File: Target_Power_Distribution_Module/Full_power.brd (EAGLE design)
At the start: 64.4 x 39.4 mm, 28 parts, among them IC1 MCP1702, Q1 NFET, Q2 PFET, Q3 NFET, Q4 PFET

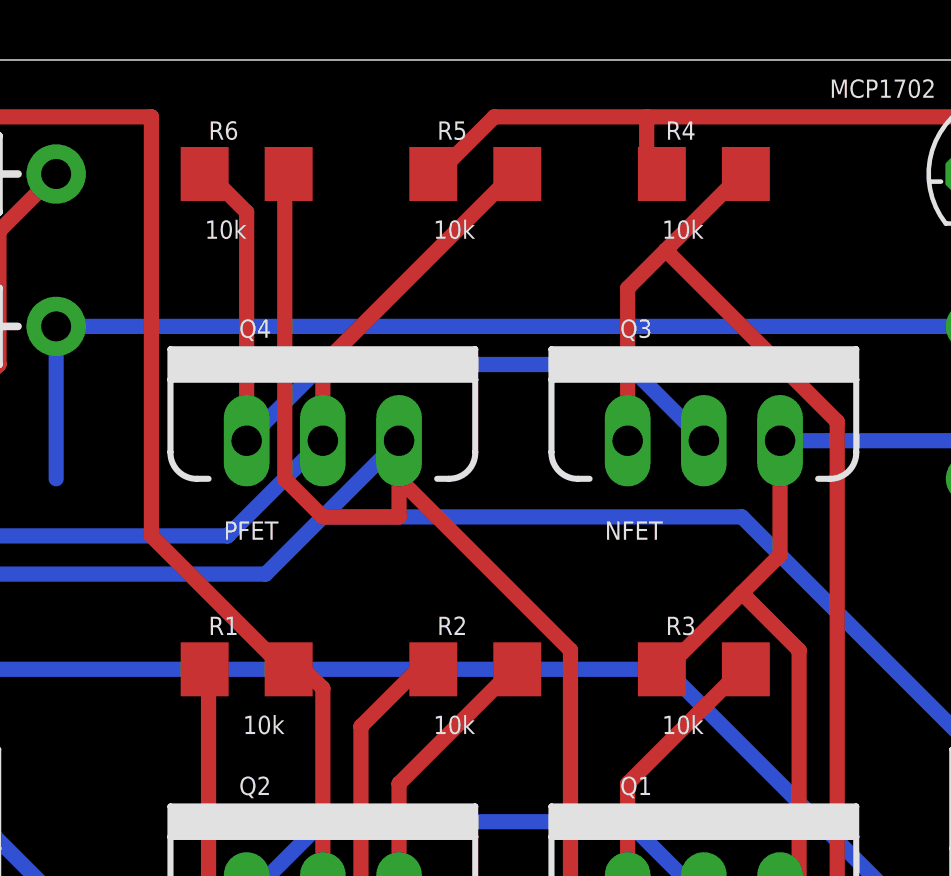
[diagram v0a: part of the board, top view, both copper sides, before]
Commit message: Cleaned sensor on full schem
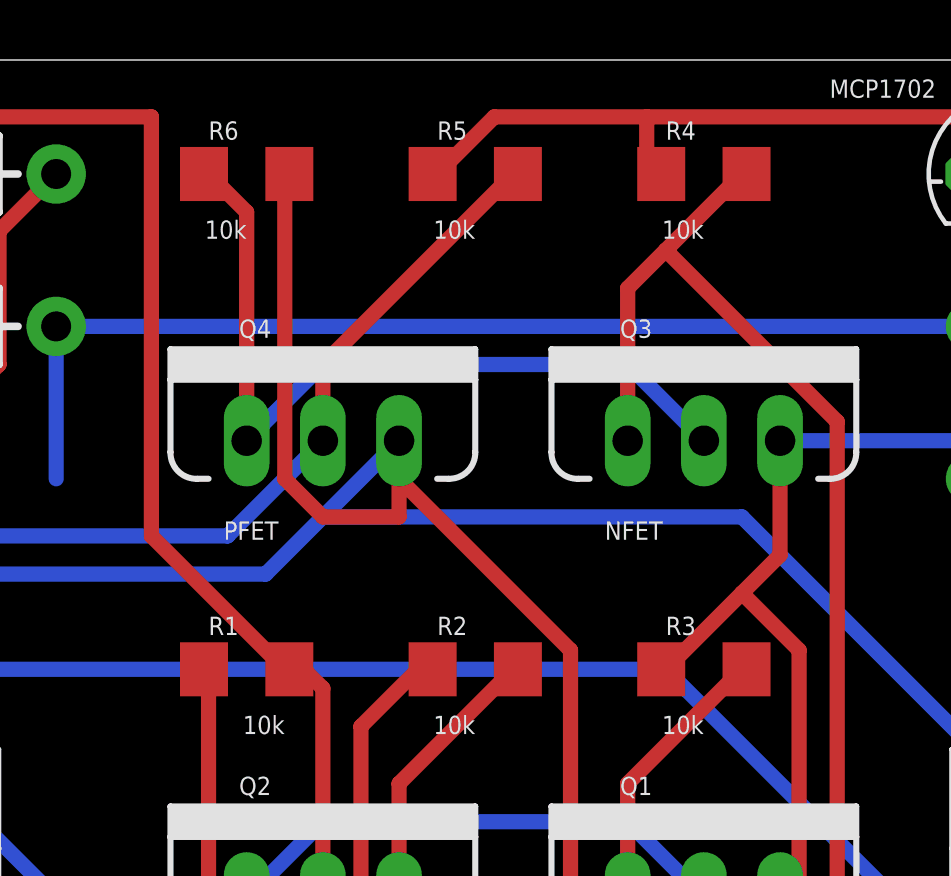
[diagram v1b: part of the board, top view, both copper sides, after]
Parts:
- R1, R2, R3, R4, R5, R6: device SparkFun-Resistors:1206 -> adafruit:R1206
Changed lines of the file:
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@@
 <attribute name="VALUE" x="33.528" y="64.008" size="0.6096" layer="25" ratio="10"/>
 </element>
-<element name="R1" library="SparkFun-Resistors" package="1206" value="10k" x="34.29" y="59.69" smashed="yes">
+<element name="R1" library="adafruit" package="R1206" value="10k" x="34.29" y="59.69" smashed="yes">
 <attribute name="NAME" x="33.02" y="60.833" size="0.6096" layer="25"/>
 <attribute name="VALUE" x="34.163" y="57.531" size="0.6096" layer="25"/>
 </element>
-<element name="R2" library="SparkFun-Resistors" package="1206" value="10k" x="41.91" y="59.69" smashed="yes">
+<element name="R2" library="adafruit" package="R1206" value="10k" x="41.91" y="59.69" smashed="yes">
 <attribute name="NAME" x="40.64" y="60.833" size="0.6096" layer="25"/>
 <attribute name="VALUE" x="40.513" y="57.531" size="0.6096" layer="25"/>
 </element>
-<element name="R3" library="SparkFun-Resistors" package="1206" value="10k" x="49.53" y="59.69" smashed="yes">
+<element name="R3" library="adafruit" package="R1206" value="10k" x="49.53" y="59.69" smashed="yes">
 <attribute name="NAME" x="48.26" y="60.833" size="0.6096" layer="25"/>
 <attribute name="VALUE" x="48.133" y="57.531" size="0.6096" layer="25"/>
 </element>
-<element name="R4" library="SparkFun-Resistors" package="1206" value="10k" x="49.53" y="76.2" smashed="yes">
+<element name="R4" library="adafruit" package="R1206" value="10k" x="49.53" y="76.2" smashed="yes">
 <attribute name="NAME" x="48.26" y="77.343" size="0.6096" layer="25"/>
 <attribute name="VALUE" x="48.133" y="74.041" size="0.6096" layer="25"/>
 </element>
-<element name="R5" library="SparkFun-Resistors" package="1206" value="10k" x="41.91" y="76.2" smashed="yes">
+<element name="R5" library="adafruit" package="R1206" value="10k" x="41.91" y="76.2" smashed="yes">
 <attribute name="NAME" x="40.64" y="77.343" size="0.6096" layer="25"/>
 <attribute name="VALUE" x="40.513" y="74.041" size="0.6096" layer="25"/>
 </element>
-<element name="R6" library="SparkFun-Resistors" package="1206" value="10k" x="34.29" y="76.2" smashed="yes">
+<element name="R6" library="adafruit" package="R1206" value="10k" x="34.29" y="76.2" smashed="yes">
 <attribute name="NAME" x="33.02" y="77.343" size="0.6096" layer="25"/>
 <attribute name="VALUE" x="32.893" y="74.041" size="0.6096" layer="25"/>
@@
 <wire x1="33.02" y1="48.26" x2="33.02" y2="59.69" width="0.508" layer="1"/>
 <wire x1="38.1" y1="43.18" x2="33.02" y2="48.26" width="0.508" layer="1"/>
-<wire x1="33.02" y1="59.69" x2="32.89" y2="59.69" width="0.508" layer="1"/>
+<wire x1="33.02" y1="59.69" x2="32.868" y2="59.69" width="0.508" layer="1"/>
 <wire x1="33.02" y1="46.355" x2="22.86" y2="46.355" width="0.508" layer="1"/>
 <wire x1="33.02" y1="48.26" x2="33.02" y2="46.355" width="0.508" layer="1"/>
@@
 <wire x1="50.8" y1="62.23" x2="48.26" y2="59.69" width="0.508" layer="1"/>
 <wire x1="52.07" y1="67.31" x2="52.07" y2="63.5" width="0.508" layer="1"/>
-<wire x1="48.26" y1="59.69" x2="48.13" y2="59.69" width="0.508" layer="1"/>
+<wire x1="48.26" y1="59.69" x2="48.108" y2="59.69" width="0.508" layer="1"/>
 <wire x1="52.705" y1="43.815" x2="52.705" y2="51.435" width="0.508" layer="1"/>
 <wire x1="53.34" y1="43.18" x2="52.705" y2="43.815" width="0.508" layer="1"/>
@@
 <wire x1="47.625" y1="78.105" x2="42.545" y2="78.105" width="0.508" layer="1"/>
 <wire x1="47.625" y1="76.2" x2="47.625" y2="78.105" width="0.508" layer="1"/>
-<wire x1="40.64" y1="76.2" x2="40.51" y2="76.2" width="0.508" layer="1"/>
-<wire x1="47.625" y1="76.2" x2="48.13" y2="76.2" width="0.508" layer="1"/>
+<wire x1="40.64" y1="76.2" x2="40.488" y2="76.2" width="0.508" layer="1"/>
+<wire x1="47.625" y1="76.2" x2="48.108" y2="76.2" width="0.508" layer="1"/>
 <wire x1="60.96" y1="71.12" x2="60.96" y2="66.04" width="0.508" layer="1"/>
 <wire x1="58.42" y1="72.39" x2="58.42" y2="76.2" width="0.508" layer="16"/>
@@
 <wire x1="34.29" y1="49.53" x2="36.83" y2="49.53" width="0.508" layer="1"/>
 <wire x1="34.29" y1="52.07" x2="34.29" y2="49.53" width="0.508" layer="1"/>
-<wire x1="40.005" y1="59.69" x2="40.51" y2="59.69" width="0.508" layer="1"/>
+<wire x1="40.005" y1="59.69" x2="40.488" y2="59.69" width="0.508" layer="1"/>
 <wire x1="46.99" y1="54.61" x2="49.53" y2="52.07" width="0.508" layer="16"/>
 <wire x1="36.83" y1="54.61" x2="46.99" y2="54.61" width="0.508" layer="16"/>
@@
 <wire x1="46.99" y1="55.88" x2="50.8" y2="59.69" width="0.508" layer="1"/>
 <wire x1="46.99" y1="52.07" x2="46.99" y2="55.88" width="0.508" layer="1"/>
-<wire x1="50.8" y1="59.69" x2="50.93" y2="59.69" width="0.508" layer="1"/>
+<wire x1="50.8" y1="59.69" x2="50.952" y2="59.69" width="0.508" layer="1"/>
 <wire x1="54.61" y1="49.53" x2="60.96" y2="43.18" width="0.508" layer="16"/>
 <wire x1="49.53" y1="49.53" x2="54.61" y2="49.53" width="0.508" layer="16"/>
@@
 <wire x1="36.83" y1="59.055" x2="36.195" y2="59.69" width="0.508" layer="1"/>
 <wire x1="36.83" y1="52.07" x2="36.83" y2="59.055" width="0.508" layer="1"/>
-<wire x1="36.195" y1="59.69" x2="35.69" y2="59.69" width="0.508" layer="1"/>
+<wire x1="36.195" y1="59.69" x2="35.712" y2="59.69" width="0.508" layer="1"/>
 <wire x1="30.48" y1="49.53" x2="24.13" y2="55.88" width="0.508" layer="16"/>
 <wire x1="34.29" y1="49.53" x2="30.48" y2="49.53" width="0.508" layer="16"/>
@@
 <wire x1="31.115" y1="64.135" x2="31.115" y2="78.105" width="0.508" layer="1"/>
 <wire x1="35.56" y1="59.69" x2="31.115" y2="64.135" width="0.508" layer="1"/>
-<wire x1="35.56" y1="59.69" x2="35.69" y2="59.69" width="0.508" layer="1"/>
+<wire x1="35.56" y1="59.69" x2="35.712" y2="59.69" width="0.508" layer="1"/>
 </signal>
 <signal name="N$5">
@@
 <wire x1="34.29" y1="74.93" x2="33.02" y2="76.2" width="0.508" layer="1"/>
 <wire x1="34.29" y1="67.31" x2="34.29" y2="74.93" width="0.508" layer="1"/>
-<wire x1="33.02" y1="76.2" x2="32.89" y2="76.2" width="0.508" layer="1"/>
+<wire x1="33.02" y1="76.2" x2="32.868" y2="76.2" width="0.508" layer="1"/>
 <wire x1="46.99" y1="69.85" x2="49.53" y2="67.31" width="0.508" layer="16"/>
 <wire x1="36.83" y1="69.85" x2="46.99" y2="69.85" width="0.508" layer="16"/>
@@
 <wire x1="39.37" y1="64.77" x2="36.83" y2="64.77" width="0.508" layer="1"/>
 <wire x1="39.37" y1="66.04" x2="39.37" y2="64.77" width="0.508" layer="1"/>
-<wire x1="35.56" y1="76.2" x2="35.69" y2="76.2" width="0.508" layer="1"/>
+<wire x1="35.56" y1="76.2" x2="35.712" y2="76.2" width="0.508" layer="1"/>
 <wire x1="23.495" y1="62.865" x2="21.59" y2="60.96" width="0.508" layer="16"/>
 <wire x1="34.925" y1="62.865" x2="23.495" y2="62.865" width="0.508" layer="16"/>
@@
 <wire x1="39.37" y1="55.88" x2="43.18" y2="59.69" width="0.508" layer="1"/>
 <wire x1="39.37" y1="52.07" x2="39.37" y2="55.88" width="0.508" layer="1"/>
-<wire x1="43.18" y1="59.69" x2="43.31" y2="59.69" width="0.508" layer="1"/>
+<wire x1="43.18" y1="59.69" x2="43.332" y2="59.69" width="0.508" layer="1"/>
 <wire x1="25.4" y1="49.53" x2="24.13" y2="48.26" width="0.508" layer="1"/>
 <wire x1="8.255" y1="46.355" x2="6.35" y2="44.45" width="0.508" layer="16"/>
@@
 <wire x1="48.26" y1="73.66" x2="50.8" y2="76.2" width="0.508" layer="1"/>
 <wire x1="46.99" y1="67.31" x2="46.99" y2="72.39" width="0.508" layer="1"/>
-<wire x1="50.8" y1="76.2" x2="50.93" y2="76.2" width="0.508" layer="1"/>
+<wire x1="50.8" y1="76.2" x2="50.952" y2="76.2" width="0.508" layer="1"/>
 <wire x1="53.975" y1="47.625" x2="58.42" y2="43.18" width="0.508" layer="1"/>
 <wire x1="53.975" y1="67.945" x2="53.975" y2="47.625" width="0.508" layer="1"/>
@@
 <wire x1="36.83" y1="69.85" x2="43.18" y2="76.2" width="0.508" layer="1"/>
 <wire x1="36.83" y1="67.31" x2="36.83" y2="69.85" width="0.508" layer="1"/>
-<wire x1="43.18" y1="76.2" x2="43.31" y2="76.2" width="0.508" layer="1"/>
+<wire x1="43.18" y1="76.2" x2="43.332" y2="76.2" width="0.508" layer="1"/>
 <wire x1="4.445" y1="65.405" x2="2.54" y2="63.5" width="0.508" layer="16"/>
 <wire x1="15.875" y1="65.405" x2="15.24" y2="65.405" width="0.508" layer="16"/>
